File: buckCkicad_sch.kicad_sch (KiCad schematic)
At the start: 23 parts, among them U6 SiC437BED-T1-GE3

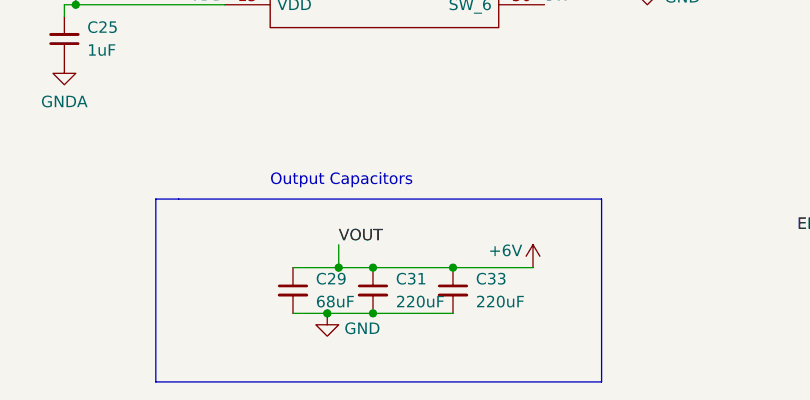
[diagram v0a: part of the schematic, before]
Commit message: commit
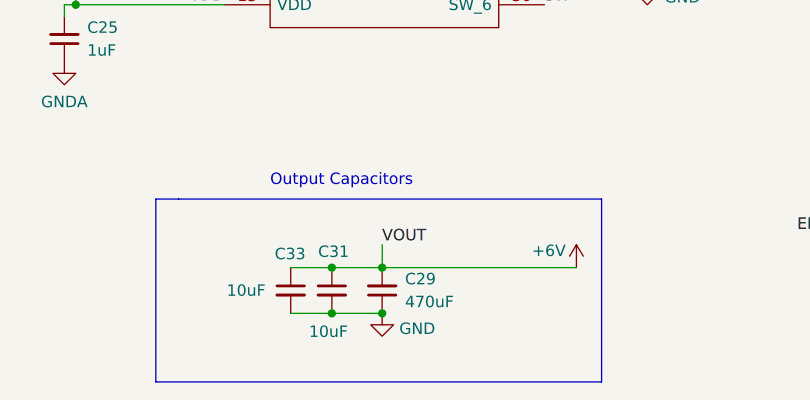
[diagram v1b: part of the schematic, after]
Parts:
- C29: value 68uF -> 470uF; footprint Capacitor_SMD:C_1206_3216Metric -> Capacitor_SMD:CP_Elec_6.3x7.7
- C31, C33: value 220uF -> 10uF; footprint Capacitor_SMD:C_1206_3216Metric -> Capacitor_SMD:C_0805_2012Metric
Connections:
- net +6V: now also C29.2; no longer C29.1
- net GND: now also C29.1; no longer C29.2
